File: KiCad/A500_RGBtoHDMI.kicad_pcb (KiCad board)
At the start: 2 copper layers, 80 x 30 mm, 3 parts, among them J1 Conn_02x20_Odd_Even, U1 Denise_MB_pins, U2 Denise_SocketOnAdapter

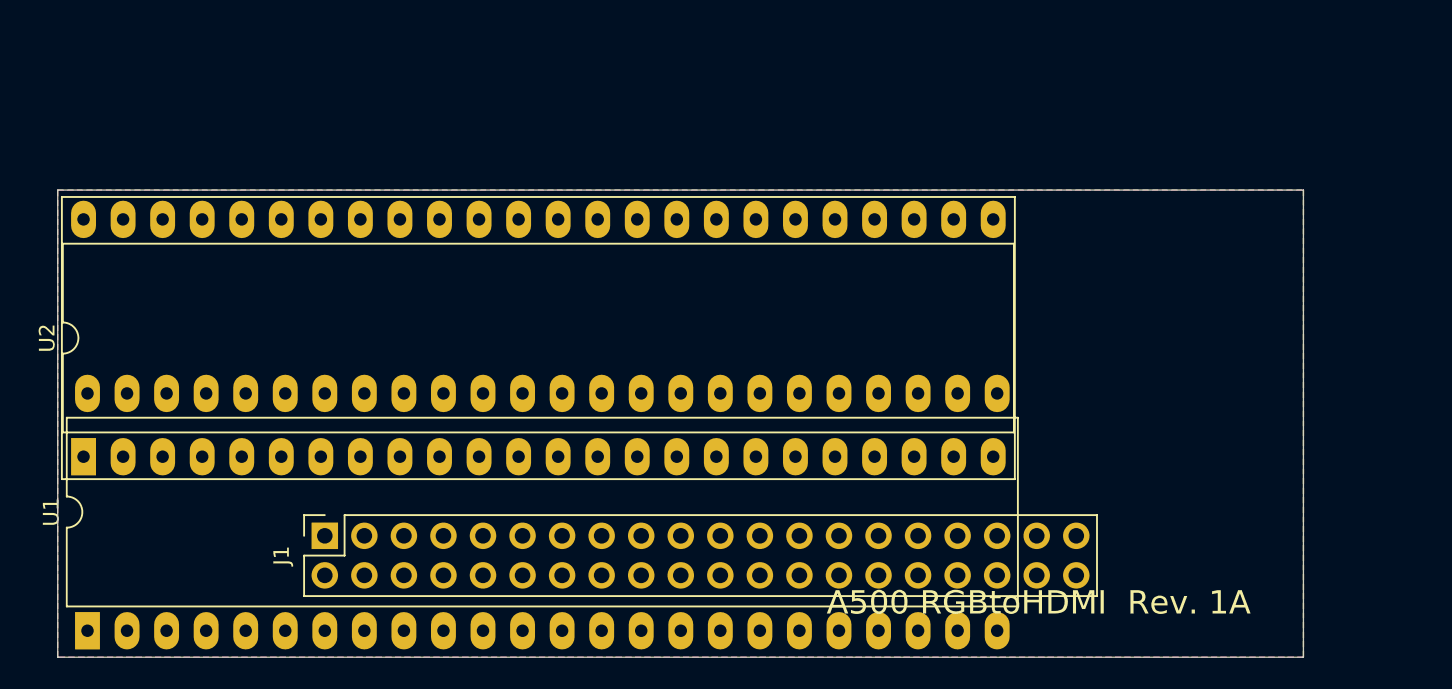
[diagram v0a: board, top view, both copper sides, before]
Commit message: improved design
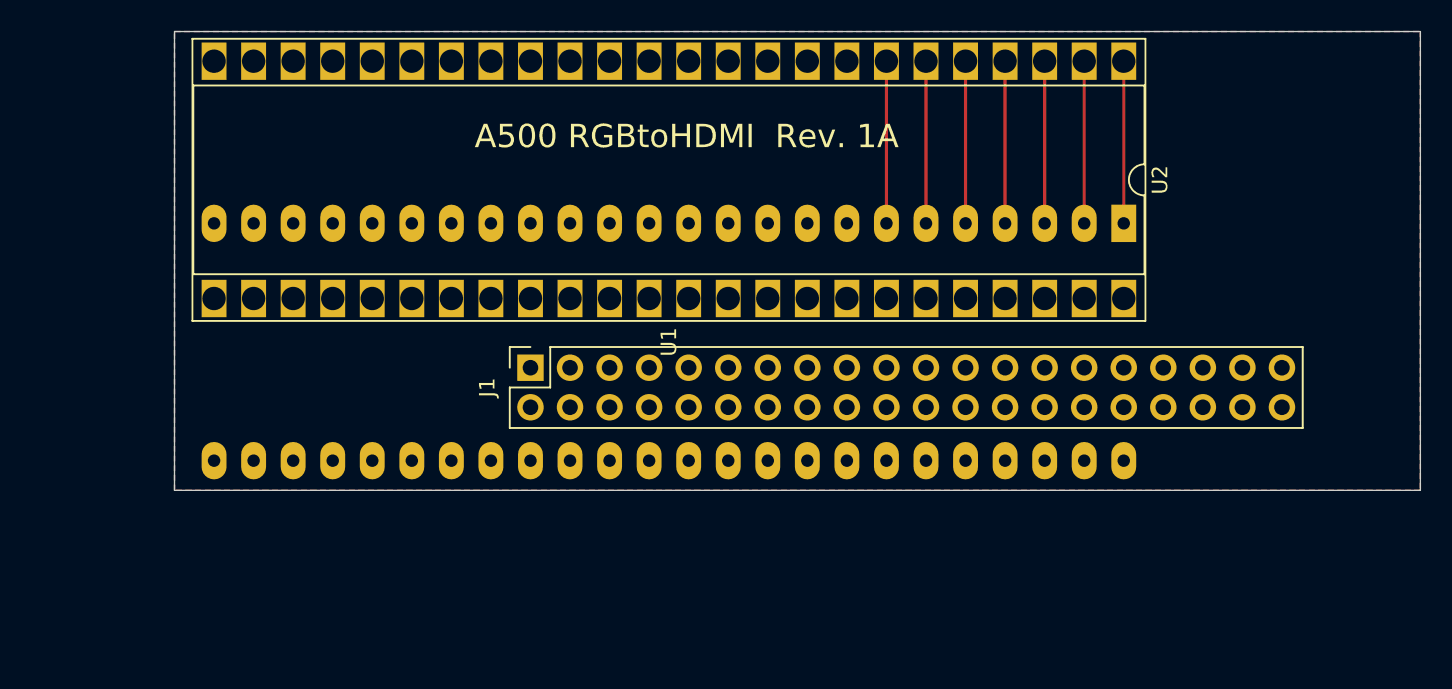
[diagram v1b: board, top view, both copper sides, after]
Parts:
- U1: value Denise_MB_pins -> Denise_MB_PinHeader
- U2: value Denise_SocketOnAdapter -> Denise_MB_PinSocket
- moved U1 71.5 mm to (188.0, 88.1), turned to 270 degrees
- moved U2 71.5 mm to (188.0, 77.7), turned to 270 degrees
- moved J1 17.1 mm to (149.9, 97.4)
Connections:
- U1 pad 1: Net-(U1-Pad1) -> D6
- U1 pad 2: Net-(U1-Pad2) -> D5
- U1 pad 3: Net-(U1-Pad3) -> D4
- U1 pad 4: Net-(U1-Pad4) -> D3
- U1 pad 5: Net-(U1-Pad5) -> D2
- U1 pad 6: Net-(U1-Pad6) -> D1
- U1 pad 7: Net-(U1-Pad7) -> D0
- U2 pad 1: Net-(U2-Pad1) -> D6
- U2 pad 2: Net-(U2-Pad2) -> D5
- U2 pad 3: Net-(U2-Pad3) -> D4
- U2 pad 4: Net-(U2-Pad4) -> D3
- U2 pad 5: Net-(U2-Pad5) -> D2
- U2 pad 6: Net-(U2-Pad6) -> D1
- U2 pad 7: Net-(U2-Pad7) -> D0
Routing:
- net D6: track 0.00 -> 10.4 mm
- net D5: track 0.00 -> 10.4 mm
- net D4: track 0.00 -> 10.4 mm
- net D3: track 0.00 -> 10.4 mm
- net D2: track 0.00 -> 10.4 mm
- net D1: track 0.00 -> 10.4 mm
- net D0: track 0.00 -> 10.4 mm
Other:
- board size 80 x 30 mm -> 80 x 29.5 mm
